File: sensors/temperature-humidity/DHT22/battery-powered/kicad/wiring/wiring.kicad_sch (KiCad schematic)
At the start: 5 parts, among them U1 arduino-pro-mini, U2 nRF24L01+

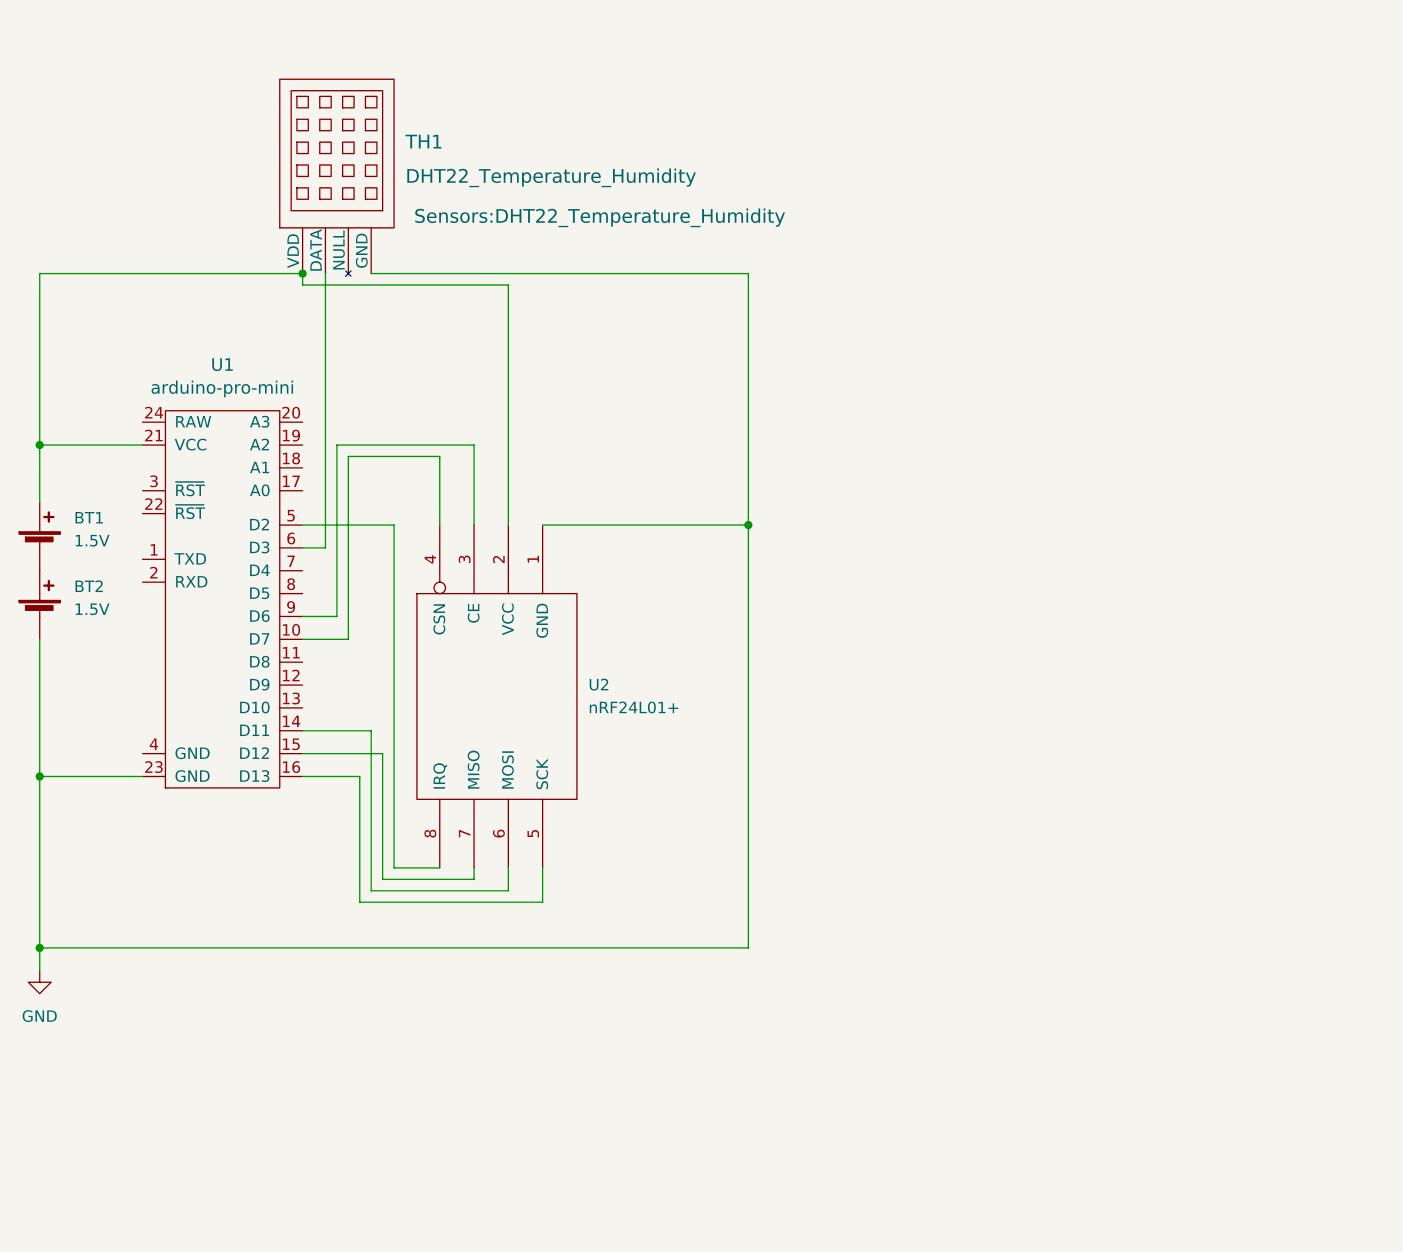
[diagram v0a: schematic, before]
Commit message: feat: better wiring
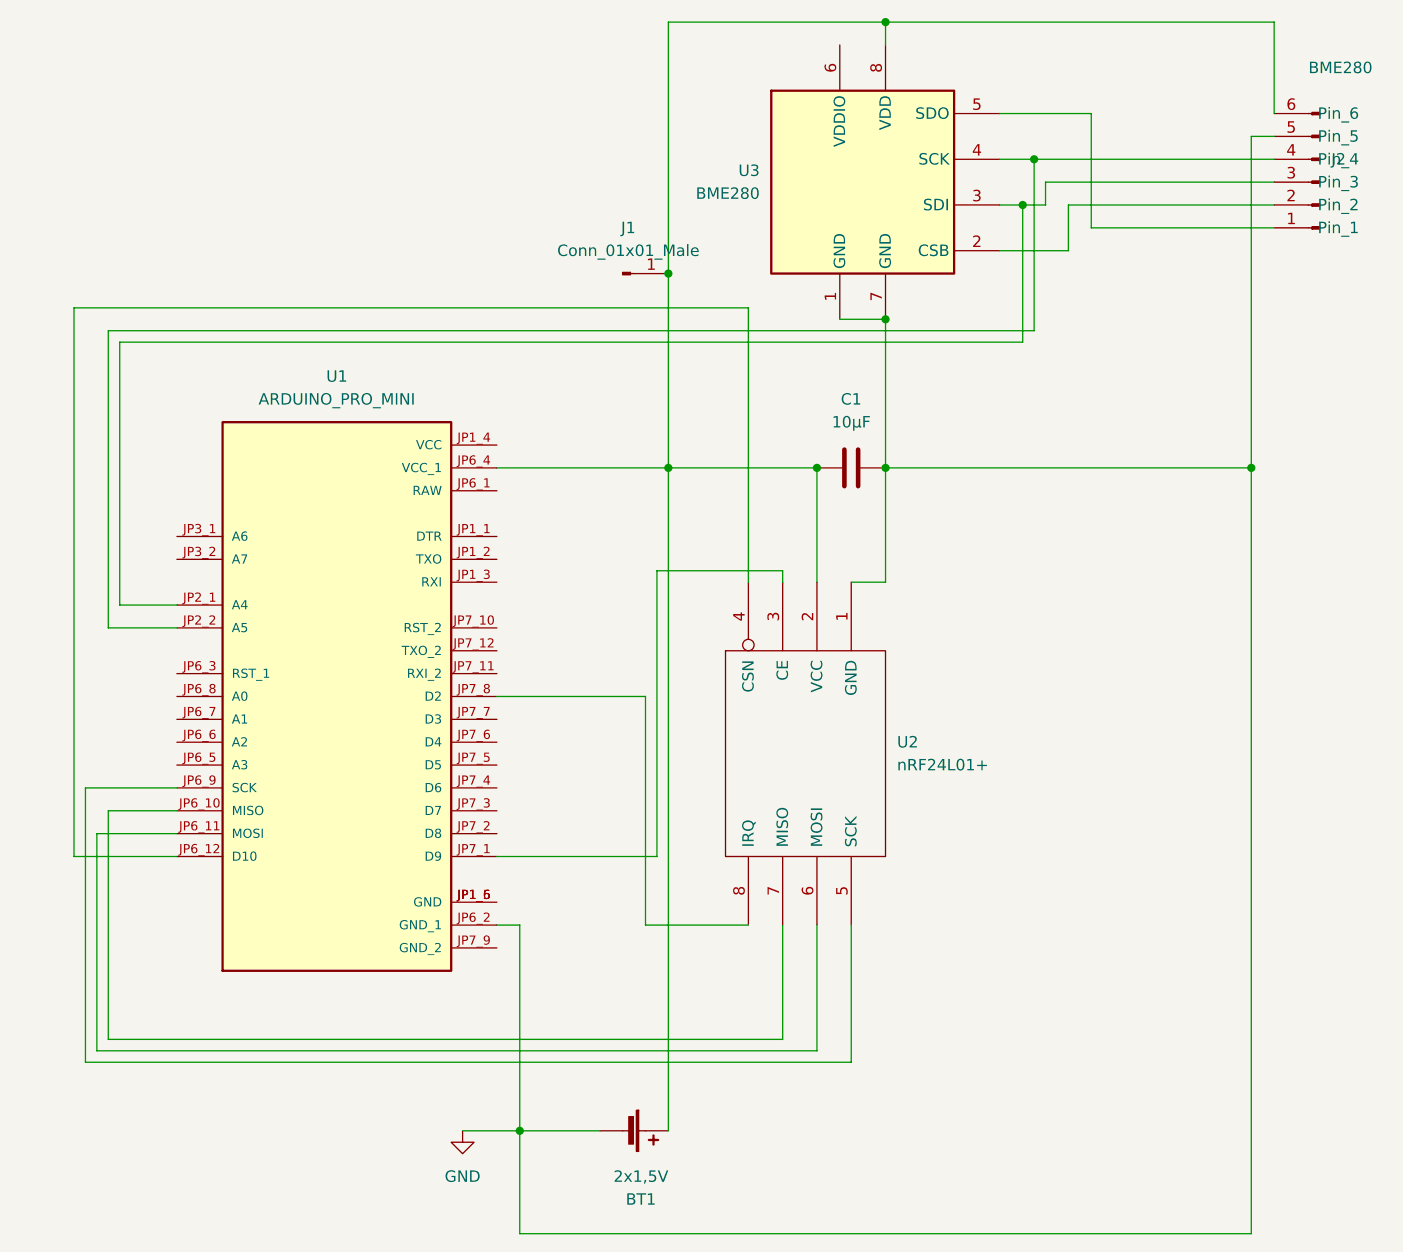
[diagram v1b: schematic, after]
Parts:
- removed BT2: 1.5V, symbol Device:Battery_Cell
- removed TH1: DHT22_Temperature_Humidity, Sensors:DHT22_Temperature_Humidity, symbol sensors:DHT22_Temperature_Humidity
- removed U1: arduino-pro-mini, symbol arduino-pro-mini:arduino-pro-mini
- added C1: 10µF, Capacitor_THT:C_Disc_D3.0mm_W1.6mm_P2.50mm, symbol Device:C
- added J1: Conn_01x01_Male, Connector_PinHeader_1.00mm:PinHeader_1x01_P1.00mm_Vertical, symbol Connector:Conn_01x01_Male
- added J2: BME280, Connector_PinHeader_2.54mm:PinHeader_1x06_P2.54mm_Vertical, symbol Connector:Conn_01x06_Male
- added U1: ARDUINO_PRO_MINI, ARDUINO_PRO_MINI:MODULE_ARDUINO_PRO_MINI, symbol ARDUINO_PRO_MINI:ARDUINO_PRO_MINI
- added U3: BME280, Package_LGA:Bosch_LGA-8_2.5x2.5mm_P0.65mm_ClockwisePinNumbering, symbol Sensor:BME280
- BT1: value 1.5V -> 2x1,5V; footprint (none) -> Battery:BatteryHolder_Keystone_2462_2xAA
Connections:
- net GND: now also BT1.2 (-), C1.2, J2.5 (Pin_5), U1.JP6_2 (GND_1), U3.1 (GND), U3.7 (GND)
- net at BT1.1 (+), U2.2 (VCC): now also C1.1, J1.1 (Pin_1), J2.6 (Pin_6), U1.JP6_4 (VCC_1), U3.8 (VDD)
- net at U2.3 (CE): now also U1.JP7_1 (D9)
- net at U2.4 (CSN): now also U1.JP6_12 (D10)
- net at U2.5 (SCK): now also U1.JP6_9 (SCK)
- net at U2.6 (MOSI): now also U1.JP6_11 (MOSI)
- net at U2.7 (MISO): now also U1.JP6_10 (MISO)
- net at U2.8 (IRQ): now also U1.JP7_8 (D2)
- new net: J2.2 (Pin_2), U3.2 (CSB)
- new net: J2.3 (Pin_3), U1.JP2_1 (A4), U3.3 (SDI)
- new net: J2.4 (Pin_4), U1.JP2_2 (A5), U3.4 (SCK)
- new net: J2.1 (Pin_1), U3.5 (SDO)
- new net: U1.JP1_5 (GND), U1.JP1_6 (GND)
